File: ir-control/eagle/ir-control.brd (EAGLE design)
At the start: 47.7 x 35.2 mm, 31 parts, among them J1 MICRO USB, J2 MICRO USB, J3 MICRO USB, Q1 DTA114EET1G (2x10K), Q3 NPN, U2 NUF2042XV6T1G, U3 LPC11U35FHI33/501, U4 MCP1754ST-3302E/CB, X1 KLBR1, Y1 12Mhz

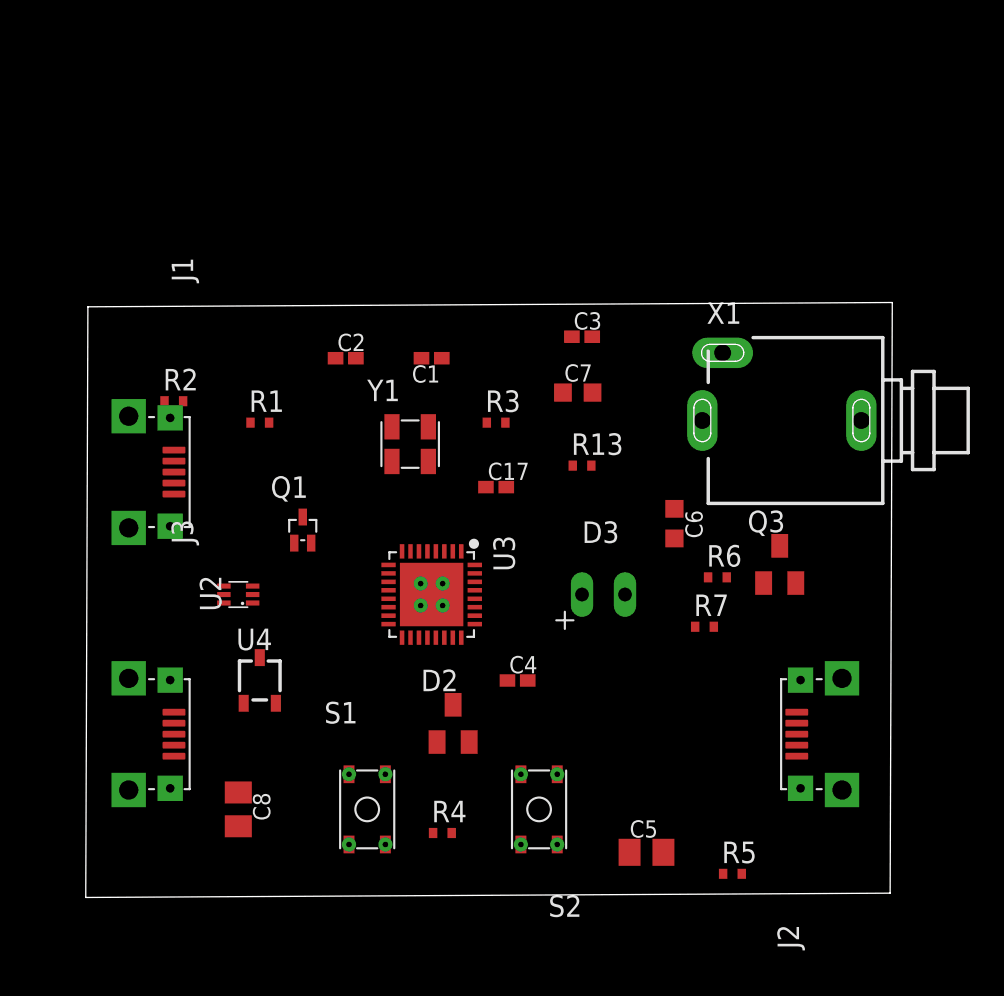
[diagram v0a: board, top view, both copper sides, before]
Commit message: Some cleanups.
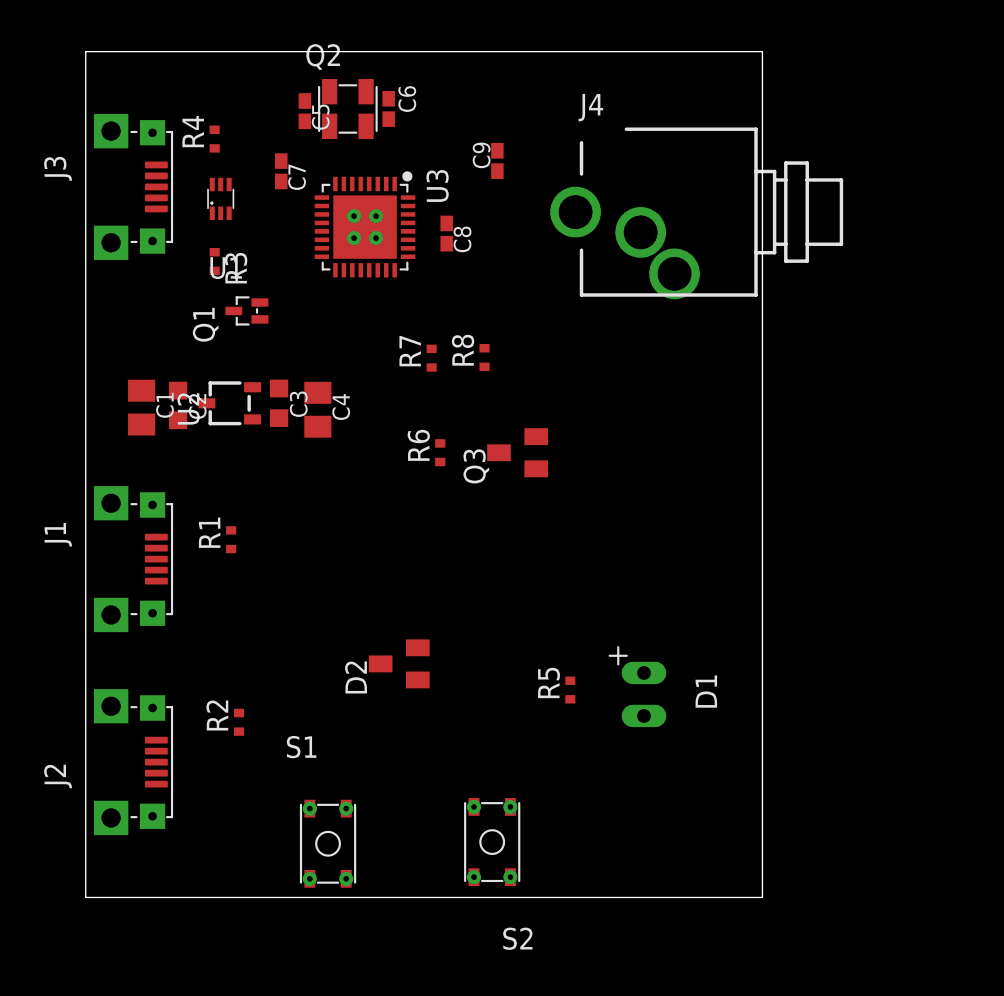
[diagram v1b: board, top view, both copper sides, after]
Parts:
- removed C17: 0.1uF, ir-control:C0402K
- removed D3: LED, ir-control:LED
- removed R13: 1K5, ir-control:R0402
- removed U4: MCP1754ST-3302E/CB, ir-control:SOT-23A
- removed X1: KLBR1, ir-control:KLBR1
- removed Y1: 12Mhz, ir-control:CRYSTAL
- added C9: 0.1uF, ir-control:C0402K
- added D1: LED, ir-control:LED
- added J4: JACKX, ir-control:JACK
- added Q2: 12Mhz, ir-control:CRYSTAL
- added R8: 10K, ir-control:R0402
- added U1: NUF2042XV6T1G, ir-control:SOT-563
- C1: value 18pF -> 10u; device ir-control:C0402K -> ir-control:C0805K
- C2: value 18pF -> 1u; device ir-control:C0402K -> ir-control:C0603K
- C3: value 0.1uF -> 1u; device ir-control:C0402K -> ir-control:C0603K
- C4: value 0.1uF -> 10u; device ir-control:C0402K -> ir-control:C0805K
- C5: value 10u -> 18pF; device ir-control:C0805K -> ir-control:C0402K
- C6: value 1u -> 18pF; device ir-control:C0603K -> ir-control:C0402K
- C7: value 1u -> 0.1uF; device ir-control:C0603K -> ir-control:C0402K
- C8: value 10u -> 0.1uF; device ir-control:C0805K -> ir-control:C0402K
- R1: value 1K5 -> 10K
- R3: value 10K -> 1K5
- R5, R7: value 10K -> 330
- R6: value 330 -> 1K5
- U2: value NUF2042XV6T1G -> MCP1754ST-3302E/CB; device ir-control:SOT-563 -> ir-control:SOT-23A
- moved C5 48.2 mm to (13.0, 46.5), turned to 270 degrees
- moved J2 43.2 mm to (1.50, 8.00), turned to 270 degrees
- moved R4 43.2 mm to (7.62, 44.8), turned to 90 degrees
- moved C8 36.2 mm to (21.3, 39.2)
- moved J3 32.4 mm to (1.50, 42.0)
- moved C6 29.8 mm to (17.9, 46.6), turned to 90 degrees
- moved R7 22.6 mm to (20.4, 31.9), turned to 90 degrees
- moved U3 22.1 mm to (16.5, 39.6)
- moved C7 21.9 mm to (11.6, 42.9), turned to 270 degrees
- moved C4 19.9 mm to (13.7, 28.8), turned to 270 degrees
- moved R2 19.4 mm to (9.06, 10.4), turned to 90 degrees
- moved R3 19.2 mm to (7.62, 37.6), turned to 270 degrees
- moved C3 18.3 mm to (11.4, 29.2), turned to 270 degrees
- moved R6 18.0 mm to (21.0, 26.3), turned to 90 degrees
- moved C1 17.4 mm to (3.30, 29.0), turned to 270 degrees
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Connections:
- net !ISP_EN: now also C9.2; no longer C17.2
- net !RESET: now also R8.1; no longer R3.1
- net +3V3: now also C7.1, C8.1, C9.1, R8.2; no longer C17.1, C3.1, C4.1, R3.2
- net +5V: now also C1.1, C2.1, J3.1, R4.1, R7.2, U1.5, U2.VIN; no longer C5.1, C6.1, J1.1, R2.1, R6.2, U2.5, U4.VIN
- net AV_SENSE: now also R2.2, U3.21; no longer R5.2
- net GND: now also D1.K, Q2.2, Q2.4, U1.2, U2.GND; no longer D3.K, U2.2, U4.GND, Y1.2, Y1.4
- net IR: now also R6.2; no longer R7.2
- net LED: now also R5.1; no longer R13.1
- net N$1: now also C5.1, Q2.3; no longer C1.1, Y1.3
- net N$12: now also J3.2, U1.4; no longer J1.2, U2.4
- net N$14: now also D1.A, R5.2; no longer D3.A, R13.2
- net N$2: now also J1.1, R1.1; no longer J2.1, R4.1
- net N$3: now also C6.1, Q2.1; no longer C2.1, Y1.1
- net N$4: now also R6.1; no longer R7.1
- net N$5: now also R3.2; no longer R1.2
- net N$6: now also J3.3, R3.1, U1.6; no longer J1.3, R1.1, U2.6
- net N$7: now also J2.1, R2.1; no longer J3.1, R5.1
- net TV_SENSE: now also R1.2, U3.19; no longer R4.2
- net USB_DM: now also U1.3; no longer U2.3
- net USB_DP: now also U1.1; no longer U2.1
- net VBUS: now also R4.2; no longer R2.2
- net VOUT: now also C3.1, C4.1, U2.VOUT; no longer C7.1, C8.1, U4.VOUT
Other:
- board size 47.7 x 35.2 mm -> 40 x 50 mm

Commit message: More progress with the layout.
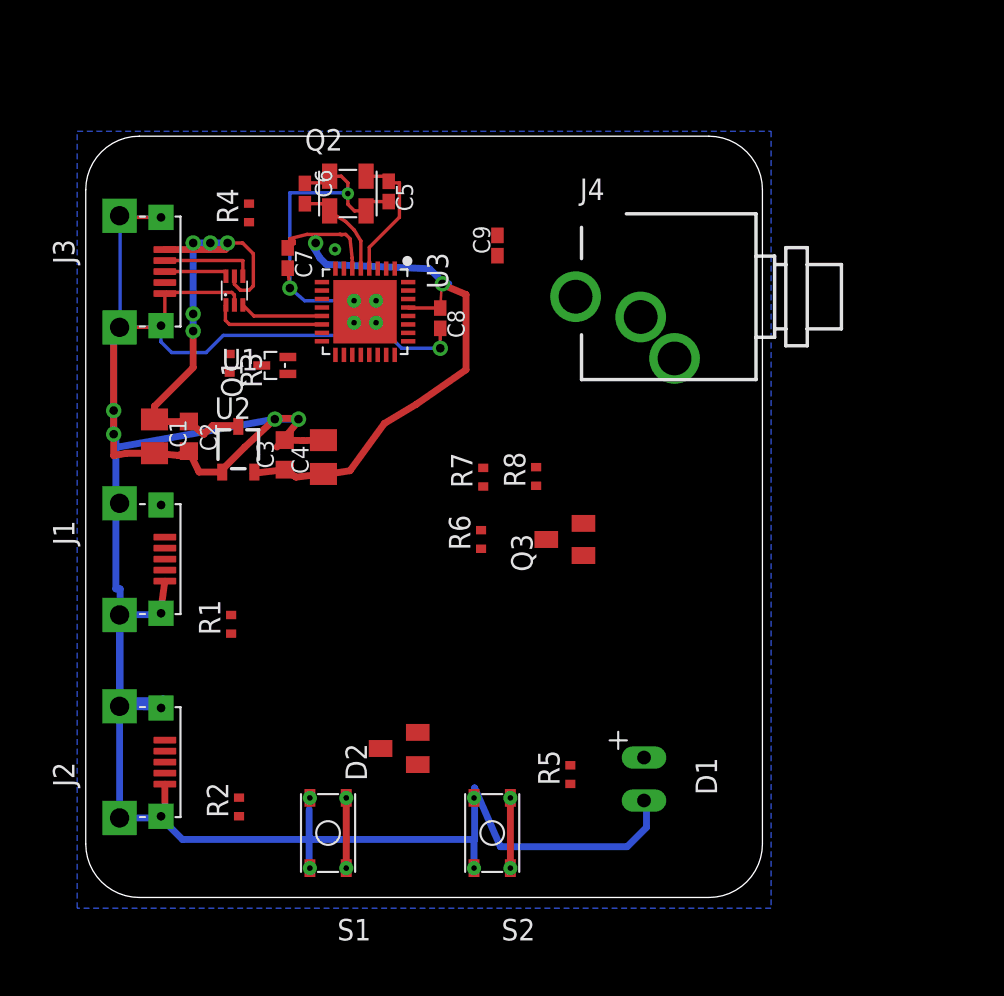
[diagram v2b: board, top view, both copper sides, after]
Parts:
- moved R7 7.66 mm to (23.5, 24.8)
- moved R8 7.66 mm to (26.6, 24.9)
- moved C6 7.04 mm to (13.0, 41.6)
- moved C5 6.86 mm to (17.9, 41.7)
- moved R3 6.08 mm to (8.51, 31.6)
- moved Q3 5.84 mm to (28.3, 21.2)
- moved R6 5.67 mm to (23.4, 21.2)
- moved U1 5.48 mm to (8.79, 35.9)
- moved C7 5.14 mm to (11.9, 37.8)
- moved J3 5.02 mm to (2.00, 37.0)
- moved C8 5.01 mm to (21.0, 34.2)
- moved R5 5.00 mm to (28.6, 7.26)
- moved C9 5.00 mm to (24.3, 38.5)
- moved D1 5.00 mm to (33.0, 7.00)
- moved D2 5.00 mm to (18.5, 8.81)
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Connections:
- removed net VOUT: C3.1, C4.1, U2.VOUT
- net +3V3: now also C3.1, C4.1, U2.VOUT
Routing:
- net GND: track 0.00 -> 200.8 mm, vias 0 -> 7
- net +3V3: track 0.00 -> 40.6 mm, vias 0 -> 2
- net +5V: track 0.00 -> 29.6 mm, vias 0 -> 5
- net N$1: track 0.00 -> 7.94 mm
- net USB_DP: track 0.00 -> 6.73 mm
- net N$3: track 0.00 -> 6.00 mm
- net N$12: track 0.00 -> 5.54 mm
- net USB_DM: track 0.00 -> 4.94 mm
- net N$16: track 0.00 -> 4.15 mm
- net !RESET: track 0.00 -> 4.15 mm
- net N$6: track 0.00 -> 3.89 mm
- net LED: track 0.00 -> 0.03 mm, vias 0 -> 1
- added copper zone on layer 16, net GND
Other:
- board size 40 x 50 mm -> 40 x 45 mm
